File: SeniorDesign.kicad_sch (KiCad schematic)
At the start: 41 parts, among them J1 USB_B_Micro, J2 Conn_01x04_Pin, J3 Conn_01x04_Pin, J4 Barrel_Jack, SW1 SW_SPDT, U1 STM32F103C8Tx, U2 AMS1117-3.3, U3 LM7812_TO220, U4 XL1509-5.0, Y1 16MHz

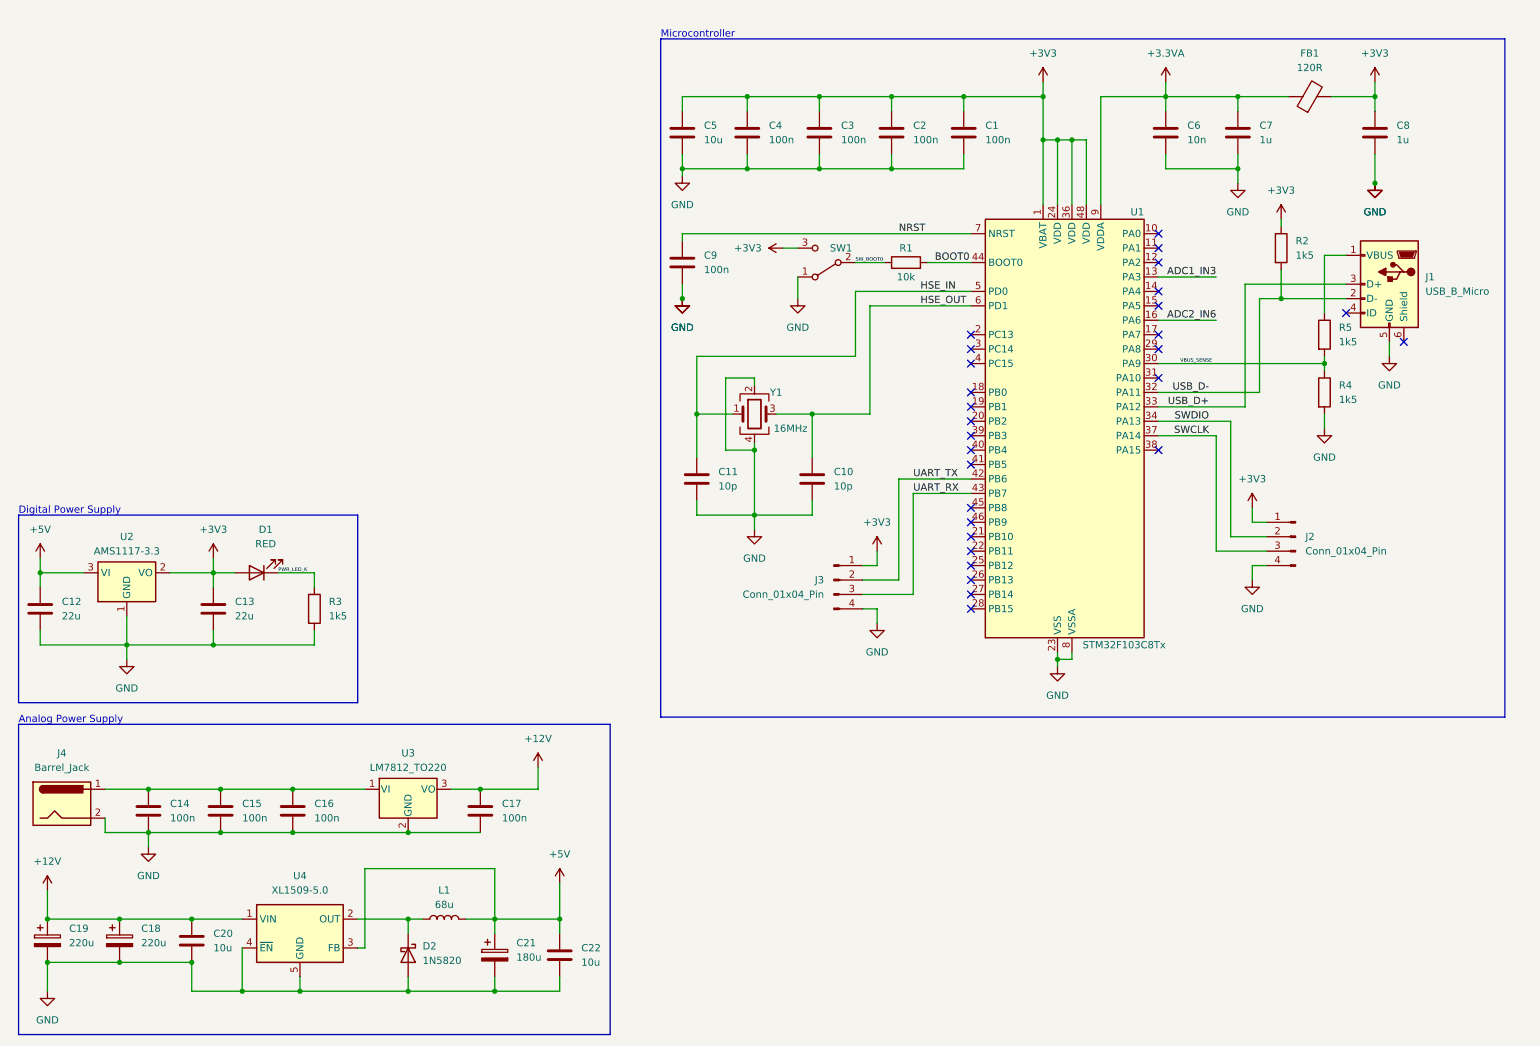
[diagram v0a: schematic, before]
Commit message: commit
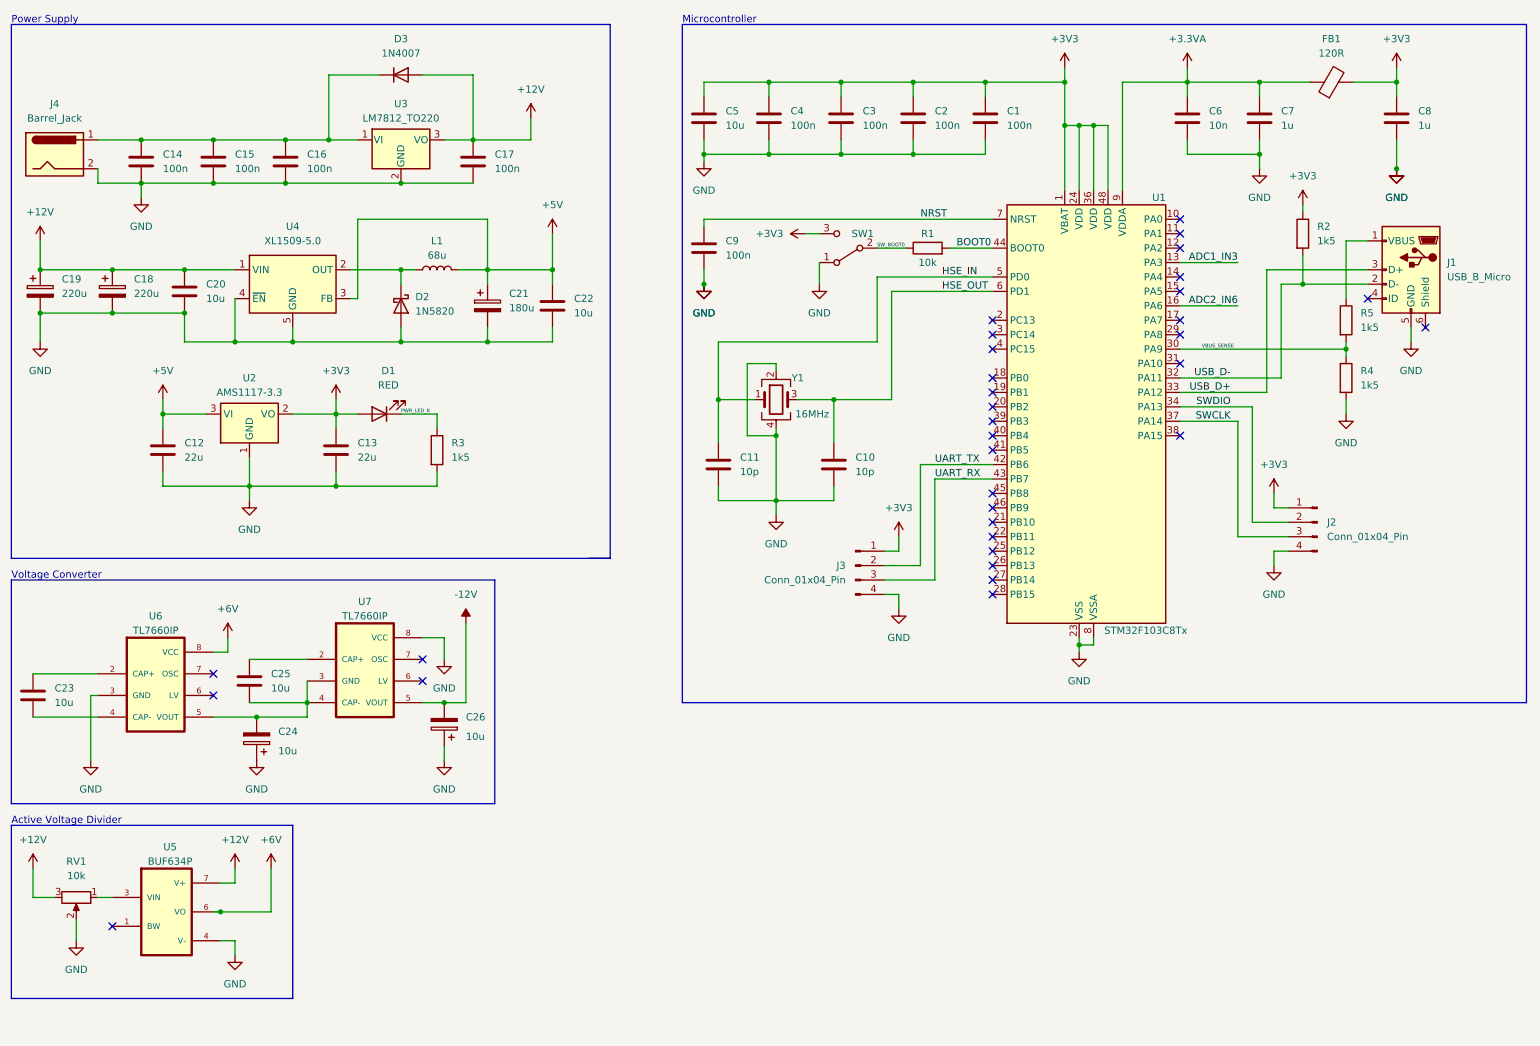
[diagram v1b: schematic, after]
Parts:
- added C23, C25: 10u, symbol Device:C
- added C24, C26: 10u, symbol Device:C_Polarized
- added D3: 1N4007, Diode_THT:D_DO-41_SOD81_P10.16mm_Horizontal, symbol Diode:1N4007
- added RV1: 10k, symbol Device:R_Potentiometer
- added U5: BUF634P, BUF634P:DIP794W45P254L959H508Q8, symbol BUF634P:BUF634P
- added U6, U7: TL7660IP, TL7660IP:DIP794W45P254L959H508Q8, symbol TL7660IP:TL7660IP
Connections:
- net +12V: now also D3.2 (A), RV1.3, U5.7 (V+)
- net GND: now also C24.1, C26.1, RV1.2, U5.4 (V-), U6.3 (GND), U7.8 (VCC)
- net at C14.1, C15.1, C16.1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: now also D3.1 (K)
- new net: C25.1, U7.2 (CAP+)
- new net: C24.2, C25.2, U6.5 (VOUT), U7.3 (GND), U7.4 (CAP-)
- new net: C23.1, U6.2 (CAP+)
- new net: C23.2, U6.4 (CAP-)
- new net: RV1.1, U5.3 (VIN)
- new net +6V: U5.6 (VO), U6.8 (VCC)
- new net -12V: C26.2, U7.5 (VOUT)
- no-connect marks 28 -> 33
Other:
- note added: "Active Voltage Divider"
- note added: "Power Supply"
- note added: "Voltage Converter"
- note removed: "Analog Power Supply"
- note removed: "Digital Power Supply"
- moved on the sheet: C1, C10, C11, C12, C13, C14, C15, C16, C17, C18, C19, C2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
